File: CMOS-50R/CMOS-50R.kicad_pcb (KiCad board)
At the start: 4 copper layers, 63.4 x 20.3 mm, 43 parts, among them J1 Conn_01x06_Male, J11 Conn_Coaxial, J21 Conn_Coaxial, J31 Conn_Coaxial, J41 Conn_Coaxial, U1 7404, U2 7404, U3 7404, U4 7404

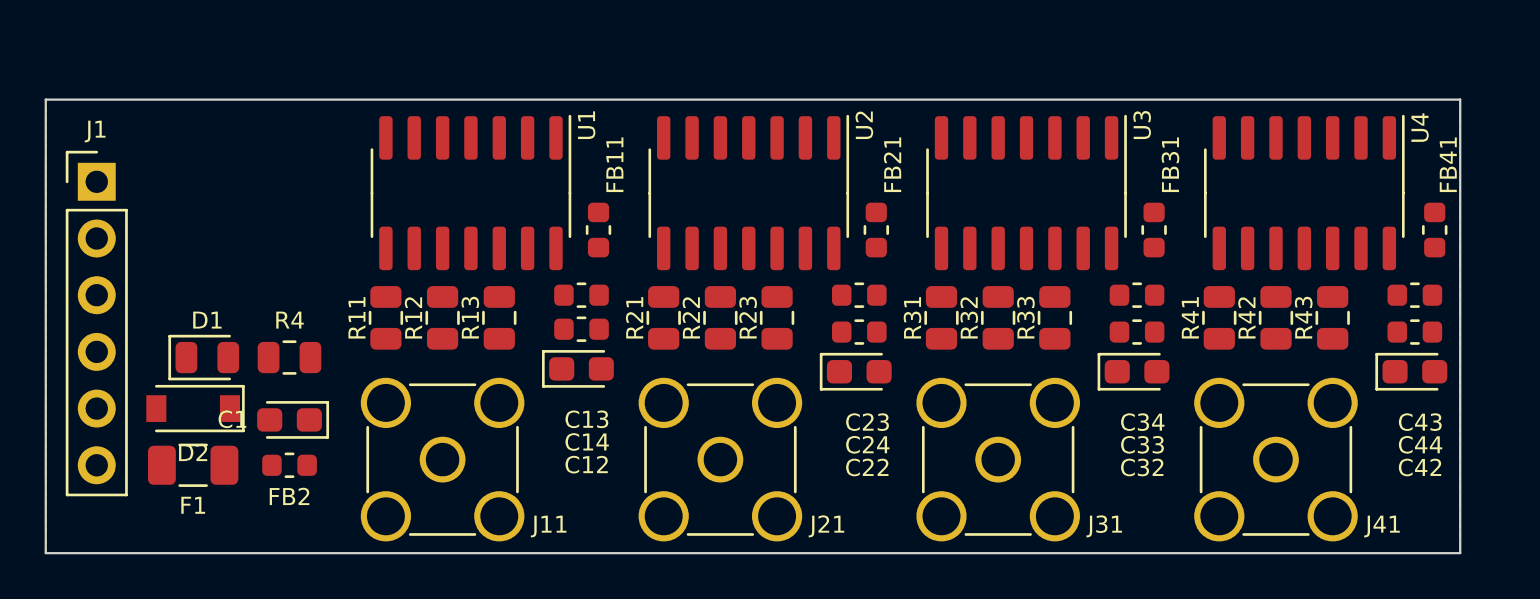
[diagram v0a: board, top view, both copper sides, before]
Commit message: layout updates
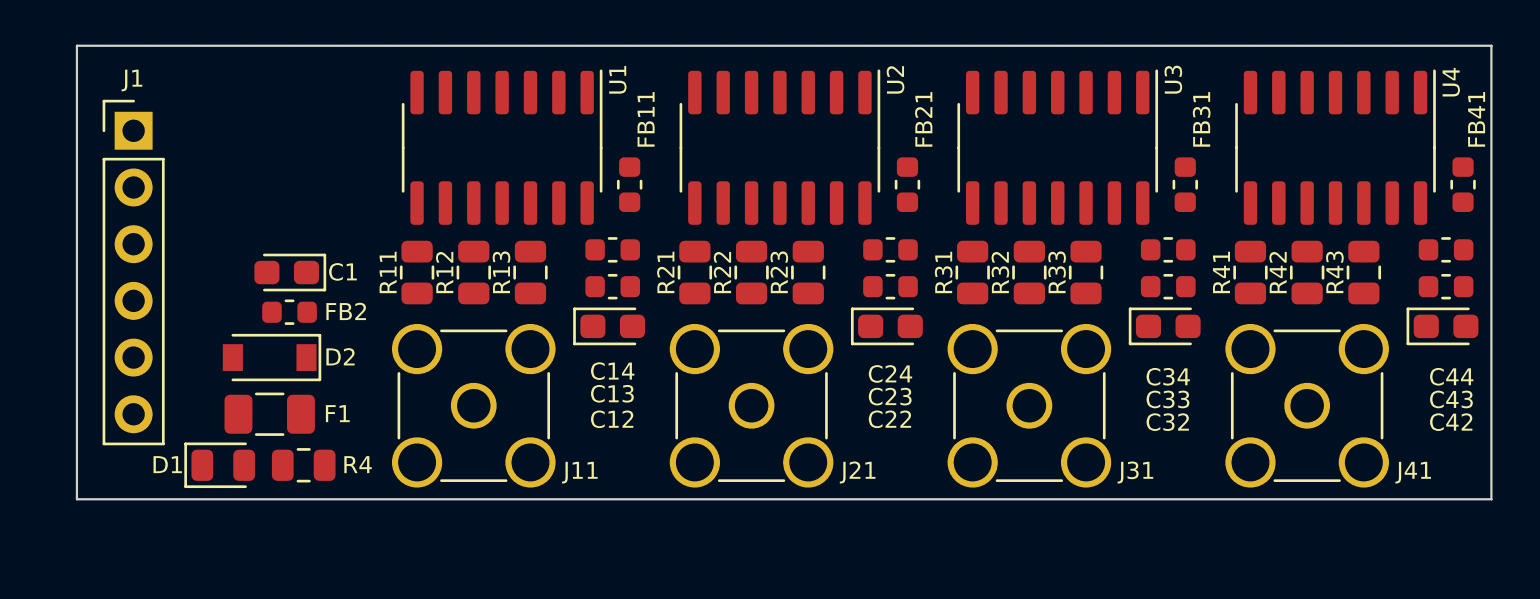
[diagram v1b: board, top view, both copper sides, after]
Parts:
- moved FB2 6.86 mm to (85.7, 67.8)
- moved C1 6.61 mm to (85.6, 66.0)
- moved D1 4.88 mm to (82.8, 74.7)
- moved R4 4.87 mm to (86.4, 74.7)
- moved D2 4.12 mm to (84.8, 69.8)
- moved F1 4.12 mm to (84.8, 72.4)
- moved C44 3.94 mm to (137.5, 65.0)
- moved C14 3.82 mm to (100.2, 65.0)
- moved J1 2.82 mm to (78.7, 59.7)
- moved J41 2.79 mm to (131.3, 72.0)
- moved J11 2.79 mm to (94.0, 72.0)
- moved J21 2.79 mm to (106.4, 72.0)
- moved J31 2.79 mm to (118.9, 72.0)
- moved R42 2.47 mm to (131.3, 66.0)
- moved FB11 2.47 mm to (101.0, 62.1)
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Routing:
- removed copper zone on GND.Cu, net GND
- removed copper zone on PWR.Cu, net VDD
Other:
- copper layers 4 -> 2
